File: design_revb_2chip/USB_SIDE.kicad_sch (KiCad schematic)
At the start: 53 parts, among them J1 USB_C_Receptacle, J2 Conn_01x08, U1 LAN7801-I/9JX, U2 TPS62162QDSGRQ1, U3 93C56A-I/P

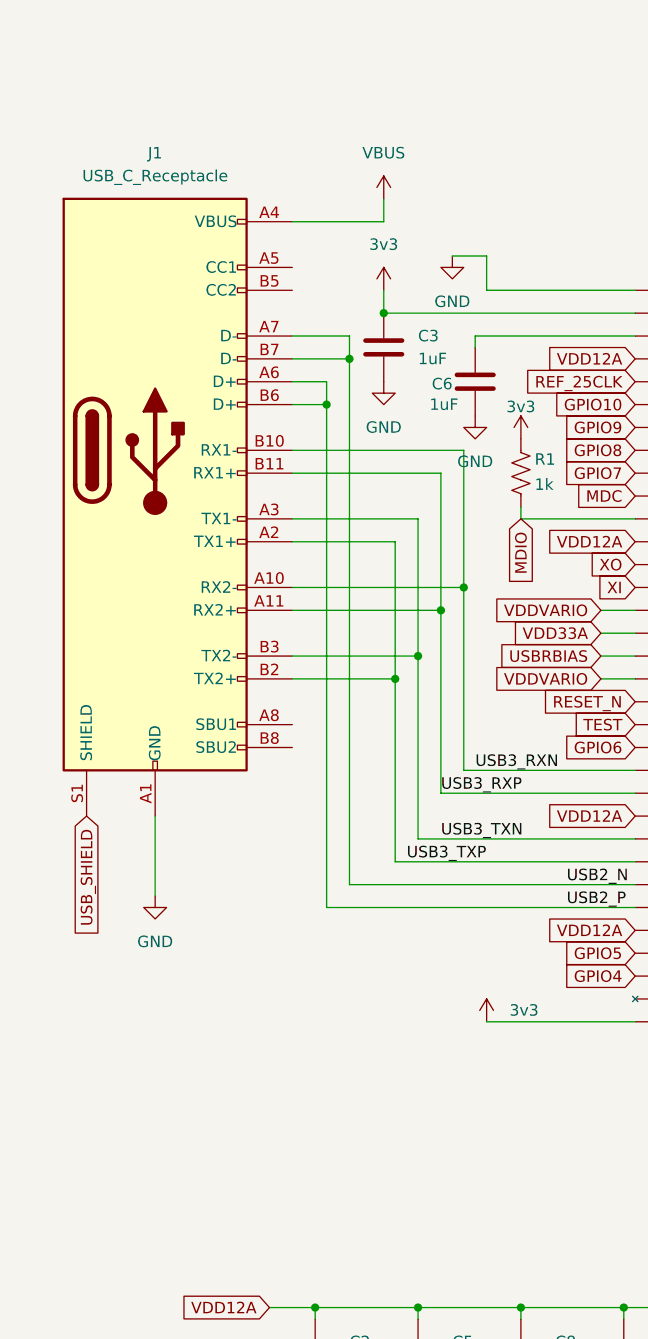
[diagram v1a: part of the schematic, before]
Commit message: Final PCB Fixes
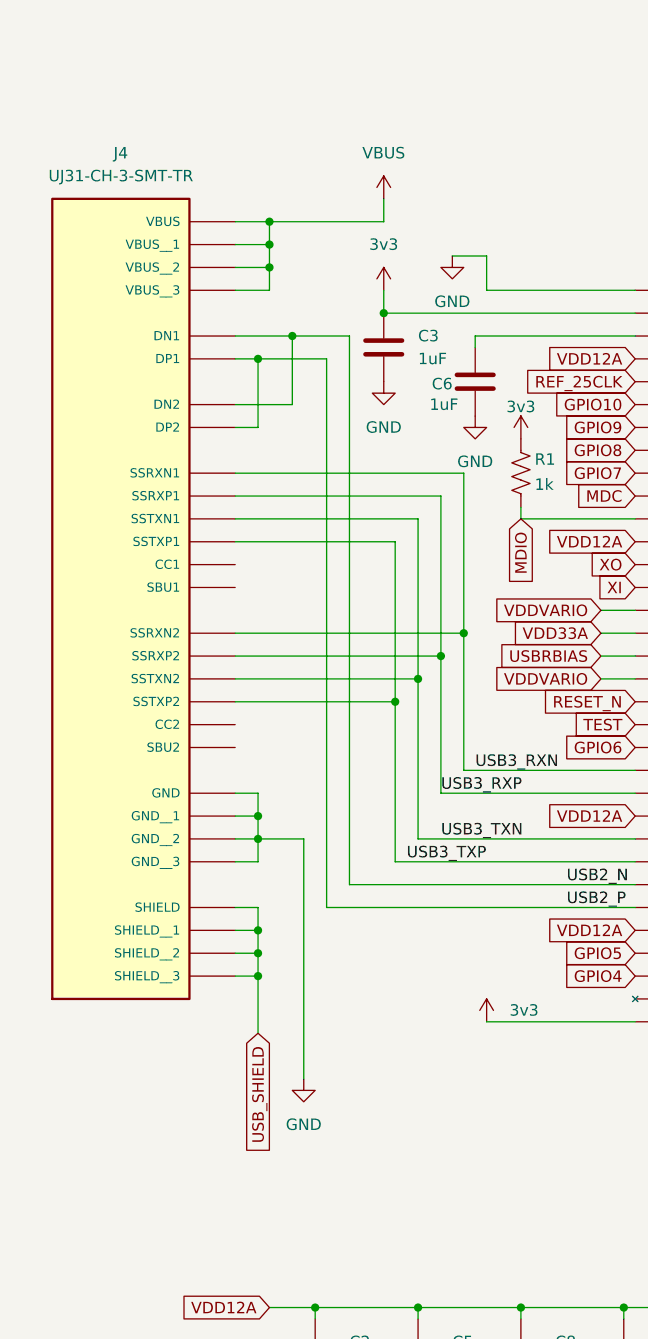
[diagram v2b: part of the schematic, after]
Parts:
- removed J1: USB_C_Receptacle, Connector_USB:USB_C_Receptacle_Molex_105450-0101, symbol Connector:USB_C_Receptacle
- added J4: UJ31-CH-3-SMT-TR, Capstone_Footprints:CUI_UJ31-CH-3-SMT-TR, symbol Capstone_Synbols:UJ31-CH-3-SMT-TR
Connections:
- net GND: now also J4.A1 (GND), J4.A12 (GND__1), J4.B1 (GND__2), J4.B12 (GND__3)
- net USB2_N: now also J4.A7 (DN1), J4.B7 (DN2)
- net USB2_P: now also J4.A6 (DP1), J4.B6 (DP2)
- net USB3_RXN: now also J4.A10 (SSRXN2), J4.B10 (SSRXN1)
- net USB3_RXP: now also J4.A11 (SSRXP2), J4.B11 (SSRXP1)
- net USB3_TXN: now also J4.A3 (SSTXN1), J4.B3 (SSTXN2)
- net USB3_TXP: now also J4.A2 (SSTXP1), J4.B2 (SSTXP2)
- net USB_SHIELD: now also J4.SH1 (SHIELD), J4.SH2 (SHIELD__1), J4.SH3 (SHIELD__2), J4.SH4 (SHIELD__3)
- net VBUS: now also J4.A4 (VBUS), J4.A9 (VBUS__1), J4.B4 (VBUS__2), J4.B9 (VBUS__3)
